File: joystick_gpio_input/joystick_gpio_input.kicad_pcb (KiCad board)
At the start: 2 copper layers, 35.3 x 46.7 mm, 27 parts, among them J1 Conn_01x06, J10 Conn_01x14, J11 Conn_01x13, J2 Conn_01x04, J3 Conn_01x15, J4 Conn_01x15, J5 Conn_01x15, J6 Conn_02x09_Odd_Even, J7 Conn_02x09_Odd_Even, J8 Conn_01x14, J9 Conn_01x13

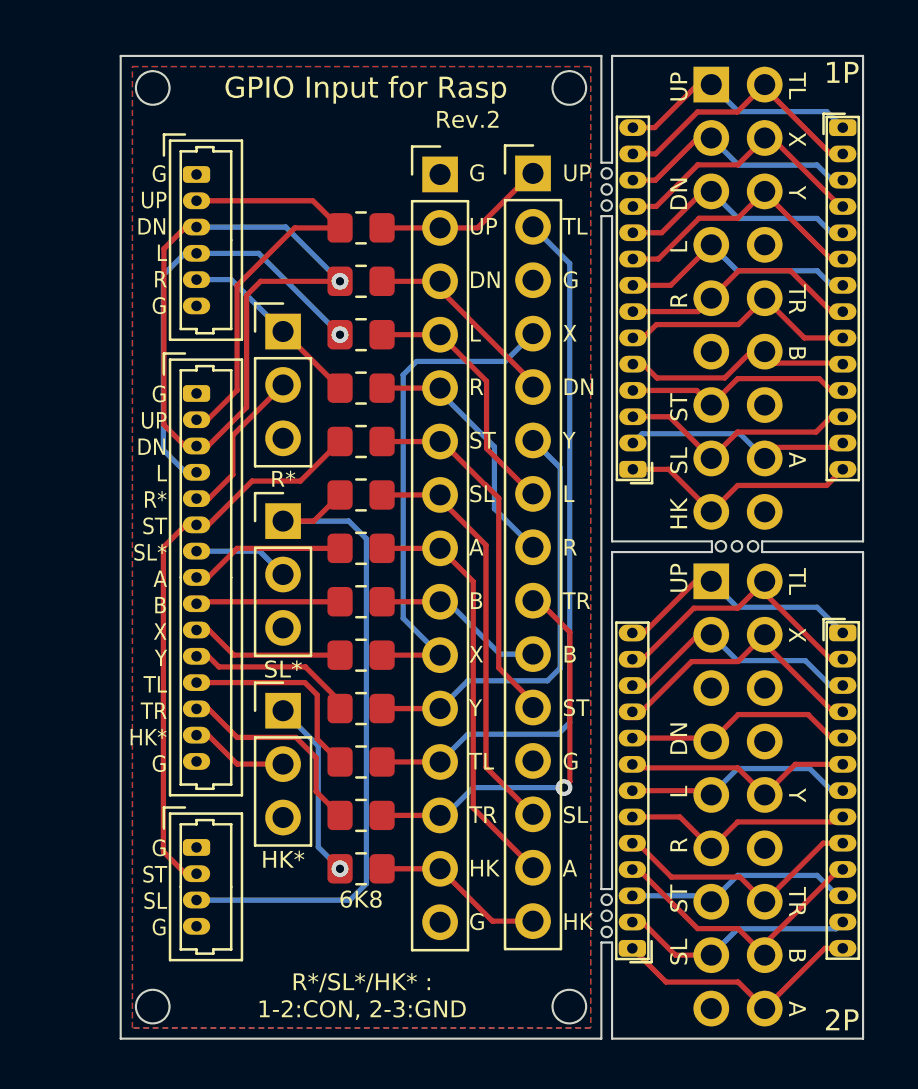
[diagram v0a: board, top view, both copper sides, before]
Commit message: Rev 2 설계
Signed-off-by: Ju, Gyeong-min <jcmh74@gmail.com>
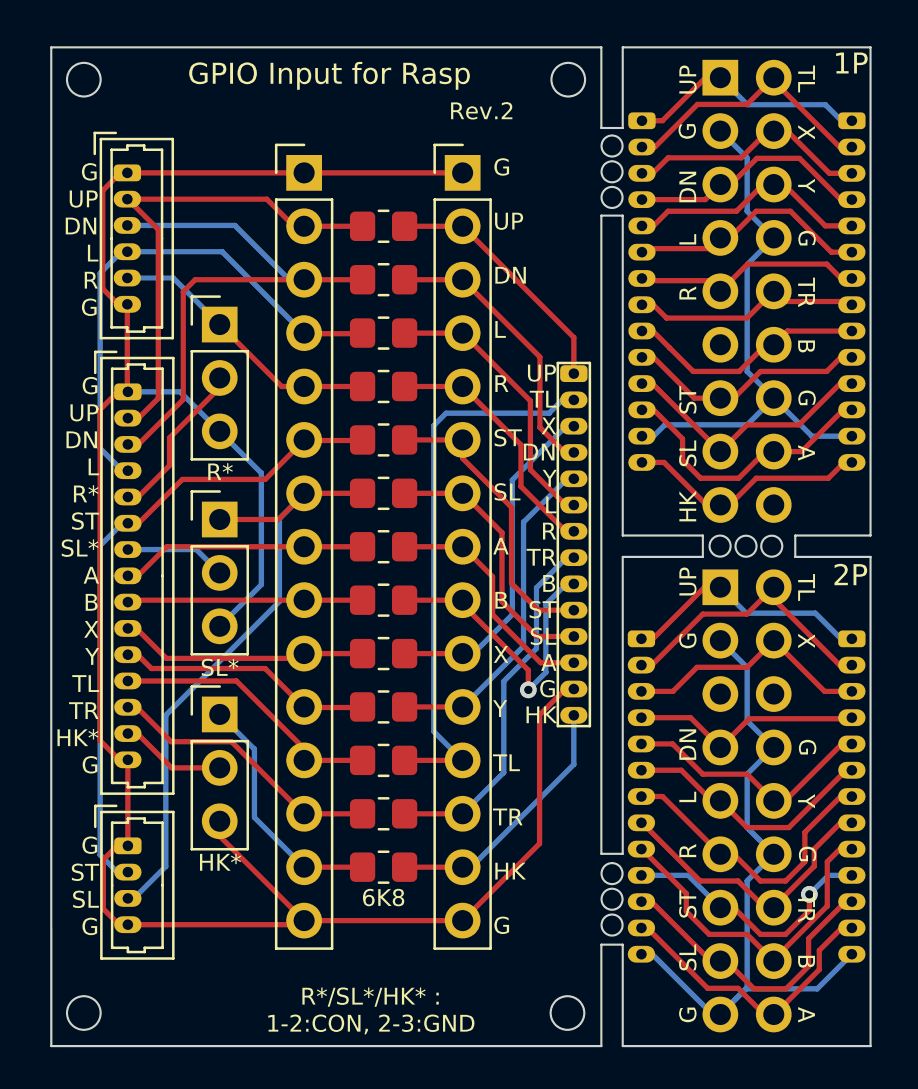
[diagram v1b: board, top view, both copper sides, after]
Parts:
- added J12: Conn_01x15, Connector_PinHeader_2.54mm:PinHeader_1x15_P2.54mm_Vertical, F.Cu at (138.3, 85.6)
- J10: footprint joystick_gpio_input_library:conn_ex_1x14_P1.25mm_Vertical -> joystick_gpio_input_library:conn_ex_1x14_P1.25mm_Vertical_Left_Labeled; moved to B.Cu
- J11: footprint joystick_gpio_input_library:conn_ex_1x13_P1.25mm_Vertical -> joystick_gpio_input_library:conn_ex_1x13_P1.25mm_Vertical_Left_Labeled; moved to B.Cu
- J5: value Conn_01x15 -> Conn_01x14; footprint Connector_PinHeader_2.54mm:PinHeader_1x15_P2.54mm_Vertical -> joystick_gpio_input_library:conn_ex_1x14_P1.25mm_Vertical_Left_Labeled
- J8: footprint joystick_gpio_input_library:conn_ex_1x14_P1.25mm_Vertical -> joystick_gpio_input_library:conn_ex_1x14_P1.25mm_Vertical_Right_Labeled; moved to B.Cu
- J9: footprint joystick_gpio_input_library:conn_ex_1x13_P1.25mm_Vertical -> joystick_gpio_input_library:conn_ex_1x13_P1.25mm_Vertical_Right_Labeled; moved to B.Cu
- moved J10 16.6 mm to (154.3, 83.1), turned to -90 degrees
- moved J11 14.7 mm to (154.3, 107.7), turned to -90 degrees
- moved J5 9.72 mm to (151.1, 95.1), turned to -90 degrees
- moved J1 3.29 mm to (129.9, 85.6)
- moved J2 3.27 mm to (129.9, 117.6)
- moved J3 3.27 mm to (129.9, 96.0)
- moved JP1 3.03 mm to (134.3, 92.8)
- moved JP3 3.02 mm to (134.3, 111.3)
- moved JP2 3.01 mm to (134.3, 102.1)
- moved J4 1.08 mm to (145.8, 85.6)
- moved R1 1.08 mm to (142.0, 88.1)
- moved R10 1.08 mm to (142.0, 111.0)
- moved R11 1.08 mm to (142.0, 113.5)
- moved R12 1.08 mm to (142.0, 116.1)
- moved R13 1.08 mm to (142.0, 118.6)
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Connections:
- J10 pad 1: /1P_HK -> /1P_UP
- J10 pad 10: /1P_DOWN -> /1P_START
- J10 pad 11: /1P_X -> /1P_SELECT
- J10 pad 12: /1P_GND -> /1P_A
- J10 pad 13: /1P_TL -> /1P_GND
- J10 pad 14: /1P_UP -> /1P_HK
- J10 pad 2: /1P_A -> /1P_TL
- J10 pad 3: /1P_SELECT -> /1P_X
- J10 pad 4: /1P_START -> /1P_DOWN
- J10 pad 5: /1P_B -> /1P_Y
- J10 pad 6: /1P_TR -> /1P_LEFT
- J10 pad 8: /1P_LEFT -> /1P_TR
- J10 pad 9: /1P_Y -> /1P_B
- J11 pad 1: /2P_A -> /2P_UP
- J11 pad 10: /2P_X -> /2P_START
- J11 pad 11: /2P_GND -> /2P_SELECT
- J11 pad 12: /2P_TL -> /2P_A
- J11 pad 13: /2P_UP -> /2P_GND
- J11 pad 2: /2P_SELECT -> /2P_TL
- J11 pad 3: /2P_START -> /2P_X
- J11 pad 4: /2P_B -> /2P_DOWN
- J11 pad 5: /2P_TR -> /2P_Y
- J11 pad 6: /2P_RIGHT -> /2P_LEFT
- J11 pad 7: /2P_LEFT -> /2P_RIGHT
- J11 pad 8: /2P_Y -> /2P_TR
- J11 pad 9: /2P_DOWN -> /2P_B
- J5 pad 10: /C_B -> /C_START
- J5 pad 11: /C_START -> /C_SELECT
- J5 pad 12: /GND -> /C_A
- J5 pad 13: /C_SELECT -> /GND
- J5 pad 14: /C_A -> /C_HK
- J5 pad 3: /GND -> /C_X
- J5 pad 4: /C_X -> /C_DOWN
- J5 pad 5: /C_DOWN -> /C_Y
- J5 pad 6: /C_Y -> /C_LEFT
- J5 pad 7: /C_LEFT -> /C_RIGHT
- J5 pad 8: /C_RIGHT -> /C_TR
- J5 pad 9: /C_TR -> /C_B
- J6 pad 14: unconnected-(J6-Pin_14-Pad14) -> /1P_GND
- J6 pad 8: unconnected-(J6-Pin_8-Pad8) -> /1P_GND
- J7 pad 12: unconnected-(J7-Pin_12-Pad12) -> /2P_GND
- J7 pad 17: unconnected-(J7-Pin_17-Pad17) -> /2P_GND
- J7 pad 8: unconnected-(J7-Pin_8-Pad8) -> /2P_GND
- J8 pad 10: /1P_B -> /1P_START
- J8 pad 11: /1P_START -> /1P_SELECT
- J8 pad 12: /1P_SELECT -> /1P_A
- J8 pad 13: /1P_A -> /1P_GND
- J8 pad 3: /1P_GND -> /1P_X
- J8 pad 4: /1P_X -> /1P_DOWN
- J8 pad 5: /1P_DOWN -> /1P_Y
- J8 pad 6: /1P_Y -> /1P_LEFT
- J8 pad 7: /1P_LEFT -> /1P_RIGHT
- J8 pad 8: /1P_RIGHT -> /1P_TR
- J8 pad 9: /1P_TR -> /1P_B
- J9 pad 10: /2P_B -> /2P_START
- J9 pad 11: /2P_START -> /2P_SELECT
- J9 pad 12: /2P_SELECT -> /2P_A
- J9 pad 13: /2P_A -> /2P_GND
- J9 pad 3: /2P_GND -> /2P_X
- J9 pad 4: /2P_X -> /2P_DOWN
- J9 pad 5: /2P_DOWN -> /2P_Y
- J9 pad 6: /2P_Y -> /2P_LEFT
- J9 pad 7: /2P_LEFT -> /2P_RIGHT
- J9 pad 8: /2P_RIGHT -> /2P_TR
- J9 pad 9: /2P_TR -> /2P_B
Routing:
- net /GND: track 0.00 -> 108.1 mm
- net /2P_GND: track 12.0 -> 33.3 mm
- net /1P_GND: track 11.6 -> 26.3 mm
- net /C_A: track 19.8 -> 11.4 mm
- net /C_TL: track 34.0 -> 26.4 mm
- net /C_X: track 23.8 -> 16.3 mm
- net /C_SELECT: track 19.8 -> 12.8 mm
- net /DOWN: track 33.4 -> 26.9 mm, vias 1 -> 0
- net /C_B: track 8.21 -> 14.5 mm, vias 0 -> 1
- net /C_Y: track 20.6 -> 16.0 mm
- net /X: track 7.32 -> 11.8 mm
- net /B: track 6.86 -> 11.3 mm
- net /RIGHT: track 8.96 -> 13.3 mm
- net /A: track 7.40 -> 11.7 mm
- net /C_HK: track 8.21 -> 12.4 mm
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- removed copper zone on B.Cu, net /GND
- removed copper zone on F.Cu, net /GND
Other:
- board size 35.3 x 46.7 mm -> 39 x 47.5 mm
- board text added: "G"
- board text removed: "UP TL G X DN Y L R TR B ST G SL A HK"
- board text removed: "UP TL G X DN Y L R TR B ST SL A"
- board text removed: "UP TL G X DN Y L R TR B ST SL A HK"
